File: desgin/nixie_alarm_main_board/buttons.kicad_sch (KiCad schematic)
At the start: 5 parts, among them IC7 AP7363-33D-13

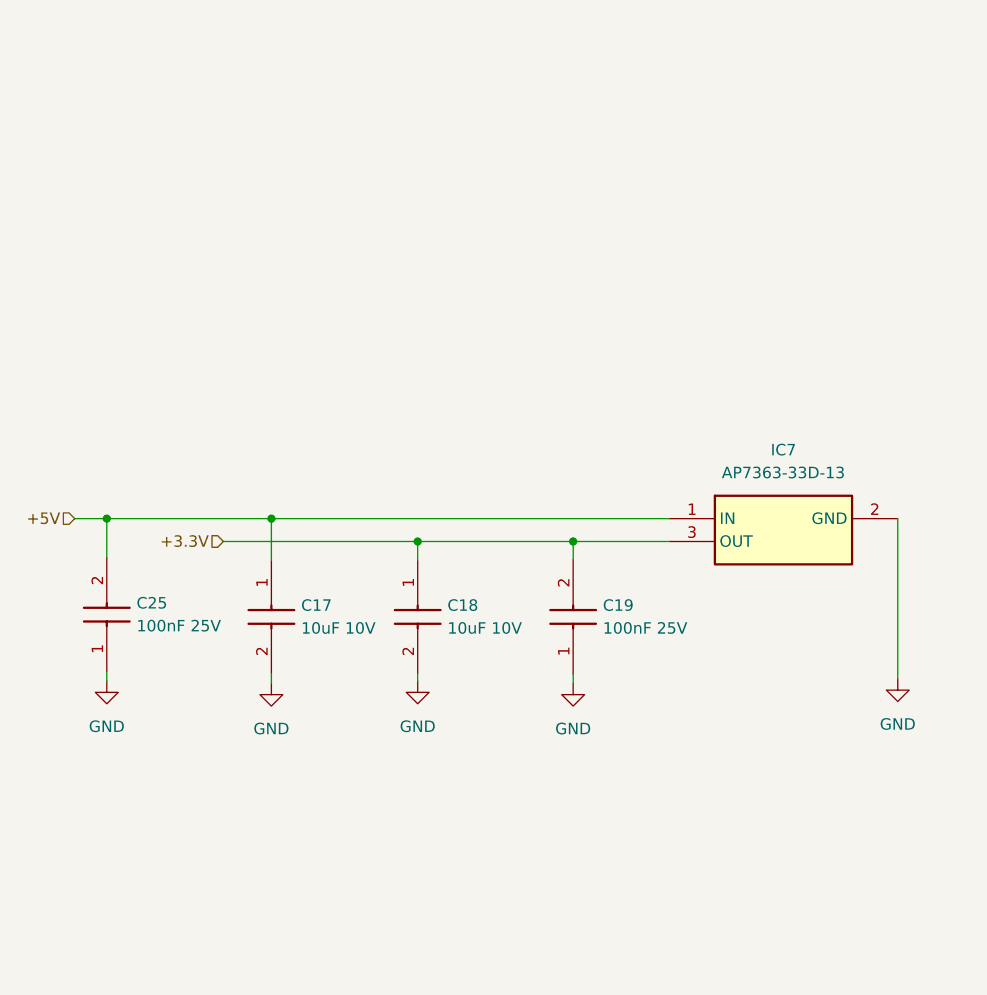
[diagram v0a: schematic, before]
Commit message: marged with board v2
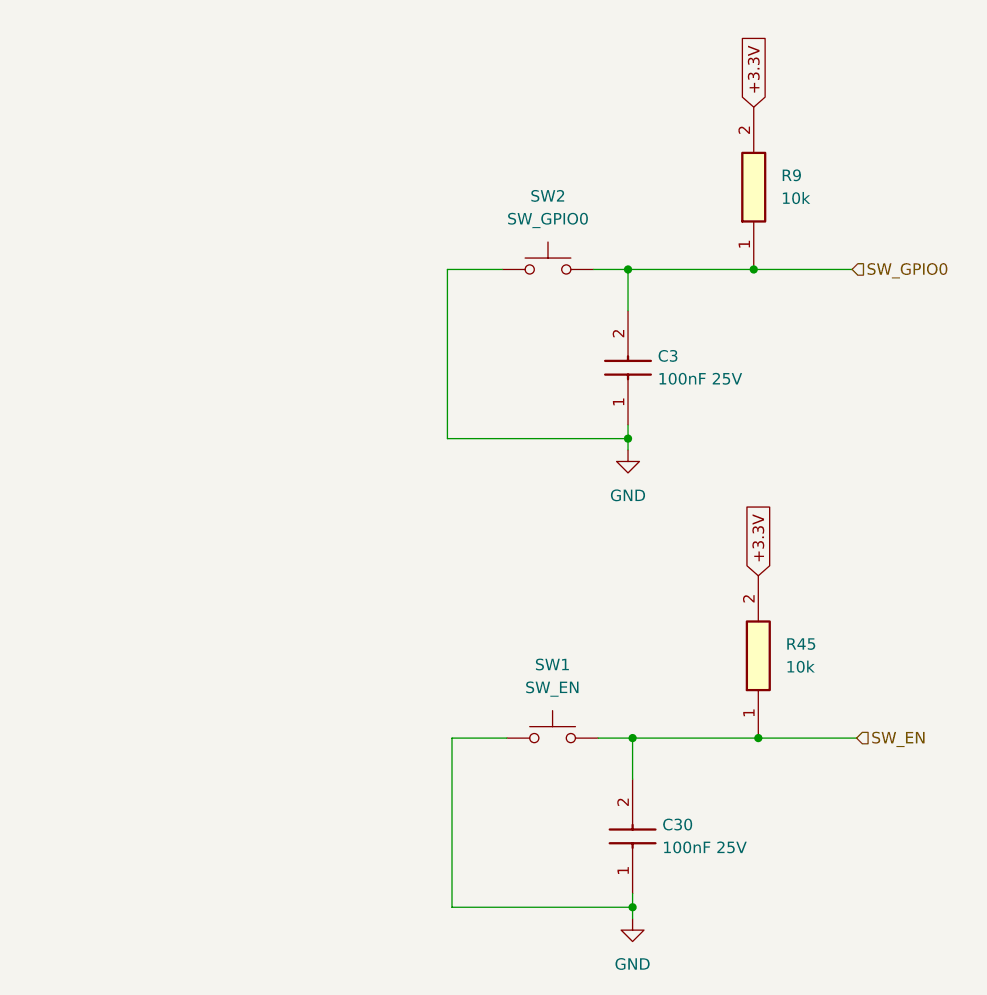
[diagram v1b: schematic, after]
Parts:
- removed C17, C18: 10uF 10V, Capacitor_SMD:C_0805_2012Metric_Pad1.18x1.45mm_HandSolder, symbol SamacSys_Parts:CL21A106KPFNNNE
- removed C19, C25: 100nF 25V, Capacitor_SMD:C_0805_2012Metric_Pad1.18x1.45mm_HandSolder, symbol SamacSys_Parts:GRM033R71E101KA01J
- removed IC7: AP7363-33D-13, AP736333D13, symbol SamacSys_Parts:AP7363-33D-13
- added C3, C30: 100nF 25V, Capacitor_SMD:C_0805_2012Metric_Pad1.18x1.45mm_HandSolder, symbol SamacSys_Parts:GRM033R71E101KA01J
- added R45, R9: 10k, Resistor_SMD:R_0805_2012Metric_Pad1.20x1.40mm_HandSolder, symbol SamacSys_Parts:ERJ-UP6D5101V
- added SW1: SW_EN, B3U1000PM, symbol Switch:SW_Push
- added SW2: SW_GPIO0, B3U1000PM, symbol Switch:SW_Push
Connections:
- net +3.3V: now also R45.2, R9.2
- net GND: now also C3.1, C30.1, SW1.1, SW2.1
- new net SW_EN: C30.2, R45.1, SW1.2
- new net SW_GPIO0: C3.2, R9.1, SW2.2
